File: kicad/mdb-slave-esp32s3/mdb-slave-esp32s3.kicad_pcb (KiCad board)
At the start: 2 copper layers, 39 x 40 mm, 45 parts, among them J1 MDB_Connector, J2 USB_C_Receptacle_USB2.0_16P, J3 Conn_01x03_Pin, J8 Conn_01x04_Pin, Q7 MMBT3904, SW1 SW_Push, U1 TLP785, U3 ESP32-S3FH4R2, U4 TLP785, U5 LM2594HVM-3.3, Y1 Crystal_GND24

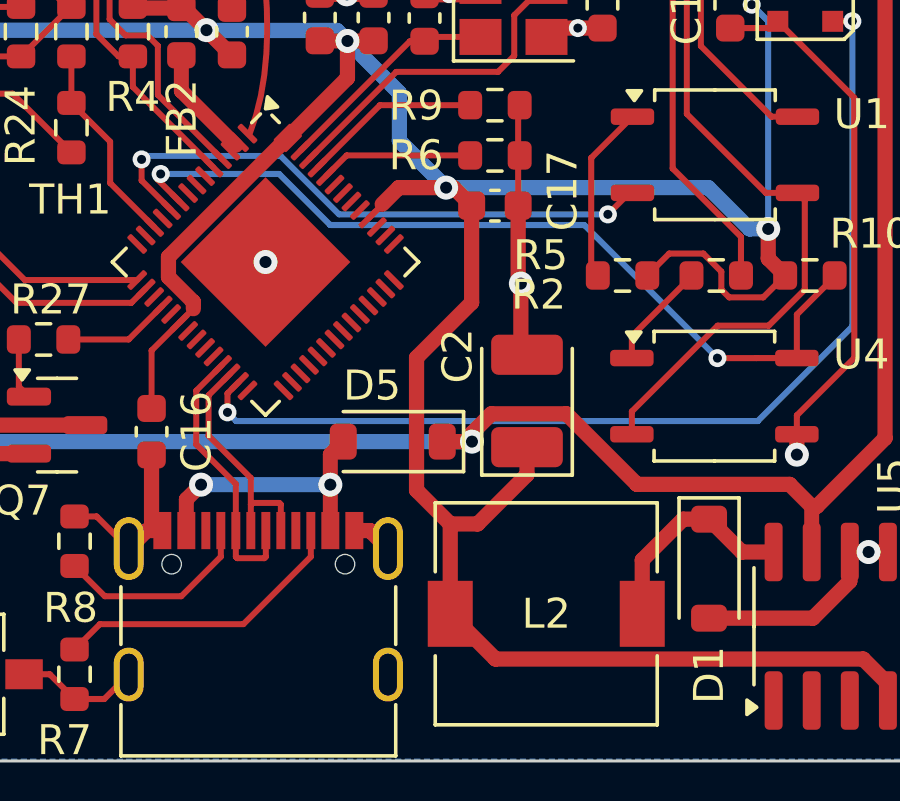
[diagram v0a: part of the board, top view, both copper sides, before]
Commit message: routing...
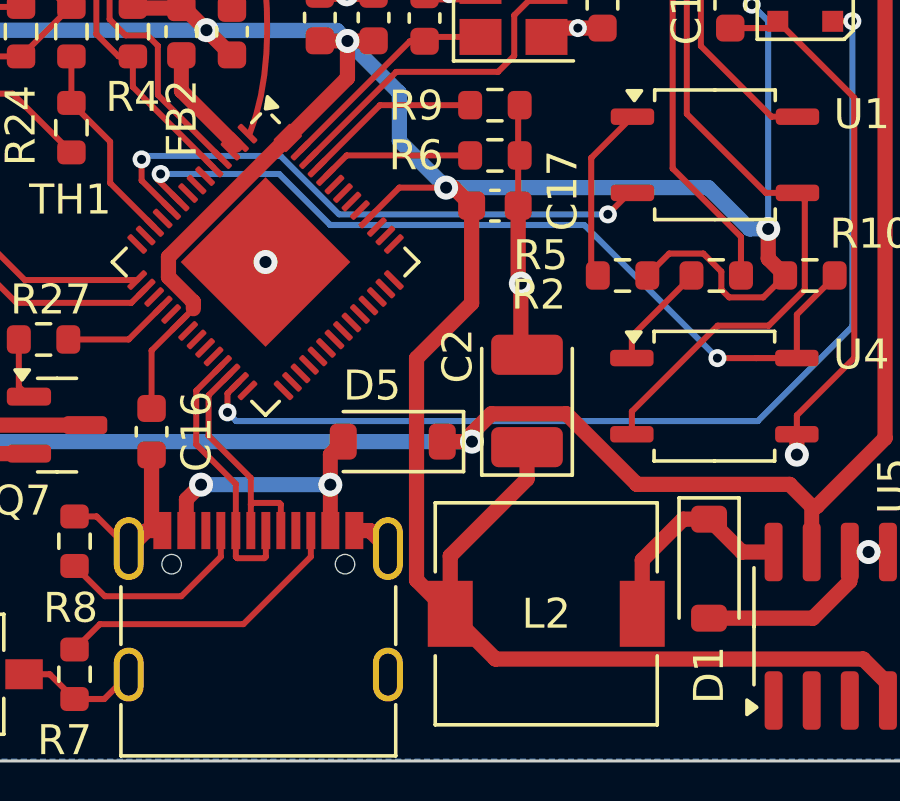
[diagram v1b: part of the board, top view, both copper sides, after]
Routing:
- net +3V3: track 125.0 -> 127.4 mm
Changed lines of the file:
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@@
+	)
+	(segment
+		(start 194.325 112.63)
+		(end 194.325 113.695)
+		(width 0.508)
+		(layer "F.Cu")
+		(net 2)
 	)
 	(segment
@@
 	)
 	(segment
-		(start 189.496806 104.550048)
-		(end 189.038427 105.008427)
-		(width 0.2032)
-		(layer "F.Cu")
-		(net 2)
-	)
-	(segment
 		(start 200.201177 106.176875)
 		(end 200.802167 106.777865)
@@
 	)
 	(segment
-		(start 192.48 107.81)
-		(end 190.6426 109.6474)
+		(start 194.325 113.695)
+		(end 191.766 116.254)
 		(width 0.508)
 		(layer "F.Cu")
@@
 	)
 	(segment
+		(start 192.48 107.83)
+		(end 192.48 104.58)
+		(width 0.508)
+		(layer "F.Cu")
+		(net 2)
+	)
+	(segment
+		(start 191.628427 103.978427)
+		(end 190.068427 103.978427)
+		(width 0.2032)
+		(layer "F.Cu")
+		(net 2)
+	)
+	(segment
 		(start 177.46 99.605)
 		(end 176.035 99.605)
@@
 	)
 	(segment
-		(start 192.48 104.58)
+		(start 190.6426 109.6674)
+		(end 192.48 107.83)
+		(width 0.508)
+		(layer "F.Cu")
+		(net 2)
+	)
+	(segment
+		(start 191.628427 103.978427)
 		(end 191.878427 103.978427)
 		(width 0.508)
@@
 		(end 202.2 107.636875)
 		(width 0.2032)
-		(layer "F.Cu")
-		(net 2)
-	)
-	(segment
-		(start 191.766 115.189)
-		(end 191.766 118.185)
-		(width 0.508)
 		(layer "F.Cu")
 		(net 2)
@@
 	)
 	(segment
-		(start 192.681 115.189)
-		(end 191.766 115.189)
+		(start 191.878427 103.978427)
+		(end 192.48 104.58)
 		(width 0.508)
 		(layer "F.Cu")
@@
 	)
 	(segment
-		(start 190.6426 109.6474)
-		(end 190.6426 114.0656)
-		(width 0.508)
-		(layer "F.Cu")
-		(net 2)
-	)
-	(segment
 		(start 202.2 107.636875)
 		(end 202.93 106.906875)
@@
 	)
 	(segment
+		(start 191.766 116.254)
+		(end 191.766 118.185)
+		(width 0.508)
+		(layer "F.Cu")
+		(net 2)
+	)
+	(segment
 		(start 179.138333 97.955)
 		(end 179.11 97.955)
 		(width 0.2)
-		(layer "F.Cu")
-		(net 2)
-	)
-	(segment
-		(start 191.878427 103.978427)
-		(end 190.051573 103.978427)
-		(width 0.508)
 		(layer "F.Cu")
 		(net 2)
@@
 	)
 	(segment
+		(start 190.068427 103.978427)
+		(end 189.038427 105.008427)
+		(width 0.2032)
+		(layer "F.Cu")
+		(net 2)
+	)
+	(segment
+		(start 190.6426 117.0616)
+		(end 190.6426 109.6674)
+		(width 0.508)
+		(layer "F.Cu")
+		(net 2)
+	)
+	(segment
 		(start 205.5324 119.6924)
 		(end 206.355 120.515)
@@
 	)
 	(segment
-		(start 194.325 112.63)
-		(end 194.325 113.545)
-		(width 0.508)
-		(layer "F.Cu")
-		(net 2)
-	)
-	(segment
-		(start 190.6426 114.0656)
-		(end 191.766 115.189)
-		(width 0.508)
-		(layer "F.Cu")
-		(net 2)
-	)
-	(segment
 		(start 177.46 96.505)
 		(end 177.545 96.505)
@@
 	)
 	(segment
+		(start 191.766 118.185)
+		(end 190.6426 117.0616)
+		(width 0.508)
+		(layer "F.Cu")
+		(net 2)
+	)
+	(segment
 		(start 200.802167 107.375885)
 		(end 201.063157 107.636875)
@@
 	)
 	(segment
-		(start 194.325 113.545)
-		(end 192.681 115.189)
-		(width 0.508)
-		(layer "F.Cu")
-		(net 2)
-	)
-	(segment
 		(start 179.11 97.955)
 		(end 177.46 99.605)
@@
 		(end 178.995 97.955)
 		(width 0.2)
-		(layer "F.Cu")
-		(net 2)
-	)
-	(segment
-		(start 192.48 104.58)
-		(end 192.48 107.81)
-		(width 0.508)
 		(layer "F.Cu")
 		(net 2)
@@
 	)
 	(segment
-		(start 189.496806 104.533194)
-		(end 189.496806 104.550048)
-		(width 0.2032)
-		(layer "F.Cu")
-		(net 2)
-	)
-	(segment
 		(start 176.035 99.605)
 		(end 175.276667 98.846667)
 		(width 0.2)
-		(layer "F.Cu")
-		(net 2)
-	)
-	(segment
-		(start 190.051573 103.978427)
-		(end 189.496806 104.533194)
-		(width 0.508)
 		(layer "F.Cu")
 		(net 2)
@@
 		(name "$teardrop_padvia$")
 		(hatch none 0.1)
-		(priority 30000)
+		(priority 30015)
 		(attr
 			(teardrop
@@
 		(polygon
 			(pts
-				(xy 194.101332 84.372878) (xy 193.742122 84.013668) (xy 192.339088 84.361698) (xy 192.124293 85.990707)
-				(xy 193.475 86.054213)
+				(xy 180.192157 120.9234) (xy 180.192157 121.1266) (xy 180.872955 121.067877) (xy 181.05 120.21)
+				(xy 180.549 119.996303)
 			)
 		)
 	)
 	(zone
-		(net 3)
-		(net_name "GND")
+		(net 27)
+		(net_name "/io11")
 		(layer "F.Cu")
 		(name "$teardrop_padvia$")
 		(hatch none 0.1)
-		(priority 30001)
+		(priority 30008)
 		(attr
 			(teardrop
@@
 		(polygon
 			(pts
-				(xy 190.507878 84.013668) (xy 190.148668 84.372878) (xy 190.775 86.054213) (xy 192.125707 85.990707)
-				(xy 191.910911 84.361698)
+				(xy 172.109084 95.731162) (xy 172.250505 95.872583) (xy 173.383528 95.446667) (xy 173.135707 94.84596)
+				(xy 172.271529 94.861609)
 			)
 		)
@@
 		(name "$teardrop_padvia$")
 		(hatch none 0.1)
-		(priority 30014)
+		(priority 30007)
 		(attr
 			(teardrop
@@
 		(polygon
 			(pts
-				(xy 180.267289 115.084605) (xy 180.123605 115.228289) (xy 180.549 116.217106) (xy 181.049707 116.010707)
-				(xy 180.78476 115.038654)
+				(xy 174.61 100.948267) (xy 174.61 100.745067) (xy 173.855671 100.265697) (xy 173.134 100.846667)
+				(xy 173.855671 101.427637)
 			)
 		)
@@
 		(name "$teardrop_padvia$")
 		(hatch none 0.1)
-		(priority 30011)
+		(priority 30006)
 		(attr
 			(teardrop
@@
 		(polygon
 			(pts
-				(xy 174.598471 96.946667) (xy 174.598471 96.746667) (xy 173.743342 96.347785) (xy 173.134 96.846667)
-				(xy 173.743342 97.345549)
+				(xy 171.92558 97.592999) (xy 172.067001 97.73442) (xy 173.327746 97.446667) (xy 173.135707 96.84596)
+				(xy 172.271529 96.729613)
 			)
 		)
@@
 		(name "$teardrop_padvia$")
 		(hatch none 0.1)
-		(priority 30007)
+		(priority 30013)
 		(attr
 			(teardrop
@@
 		(polygon
 			(pts
-				(xy 174.61 100.948267) (xy 174.61 100.745067) (xy 173.855671 100.265697) (xy 173.134 100.846667)
-				(xy 173.855671 101.427637)
+				(xy 188.730421 115.156) (xy 188.730421 115.664) (xy 189.189 116.286434) (xy 189.69 116.01) (xy 189.287099 115.16838)
 			)
 		)
@@
 	)
 	(zone
-		(net 27)
-		(net_name "/io11")
+		(net 12)
+		(net_name "/mdb_master_receive")
 		(layer "F.Cu")
 		(name "$teardrop_padvia$")
 		(hatch none 0.1)
-		(priority 30008)
+		(priority 30003)
 		(attr
 			(teardrop
@@
 		(polygon
 			(pts
-				(xy 172.109084 95.731162) (xy 172.250505 95.872583) (xy 173.383528 95.446667) (xy 173.135707 94.84596)
-				(xy 172.271529 94.861609)
+				(xy 189.792438 89.763983) (xy 189.651017 89.622562) (xy 188.139088 89.861698) (xy 187.924293 91.490707)
+				(xy 189.275 91.554214)
 			)
 		)
 	)
 	(zone
-		(net 27)
-		(net_name "/io11")
+		(net 2)
+		(net_name "+3V3")
 		(layer "F.Cu")
 		(name "$teardrop_padvia$")
 		(hatch none 0.1)
-		(priority 30009)
+		(priority 30010)
 		(attr
 			(teardrop
@@
 		(polygon
 			(pts
-				(xy 174.598471 94.946667) (xy 174.598471 94.746667) (xy 173.743342 94.347785) (xy 173.134 94.846667)
-				(xy 173.743342 95.345549)
+				(xy 174.598471 98.946667) (xy 174.598471 98.746667) (xy 173.743342 98.347785) (xy 173.134 98.846667)
+				(xy 173.743342 99.345549)
 			)
 		)
 	)
 	(zone
-		(net 23)
-		(net_name "/io10")
+		(net 3)
+		(net_name "GND")
 		(layer "F.Cu")
 		(name "$teardrop_padvia$")
 		(hatch none 0.1)
-		(priority 30006)
+		(priority 30012)
 		(attr
 			(teardrop
@@
 		(polygon
 			(pts
-				(xy 171.92558 97.592999) (xy 172.067001 97.73442) (xy 173.327746 97.446667) (xy 173.135707 96.84596)
-				(xy 172.271529 96.729613)
+				(xy 182.007579 115.664) (xy 182.007579 115.156) (xy 181.4509 115.16838) (xy 181.048 116.01) (xy 181.549 116.286434)
 			)
 		)
 	)
 	(zone
-		(net 2)
-		(net_name "+3V3")
+		(net 3)
+		(net_name "GND")
 		(layer "F.Cu")
 		(name "$teardrop_padvia$")
 		(hatch none 0.1)
-		(priority 30010)
+		(priority 30001)
 		(attr
 			(teardrop
@@
 		(polygon
 			(pts
-				(xy 174.598471 98.946667) (xy 174.598471 98.746667) (xy 173.743342 98.347785) (xy 173.134 98.846667)
-				(xy 173.743342 99.345549)
+				(xy 190.507878 84.013668) (xy 190.148668 84.372878) (xy 190.775 86.054213) (xy 192.125707 85.990707)
+				(xy 191.910911 84.361698)
 			)
 		)
@@
 		(name "$teardrop_padvia$")
 		(hatch none 0.1)
-		(priority 30012)
+		(priority 30000)
 		(attr
 			(teardrop
@@
 		(polygon
 			(pts
-				(xy 182.007579 115.664) (xy 182.007579 115.156) (xy 181.4509 115.16838) (xy 181.048 116.01) (xy 181.549 116.286434)
+				(xy 194.101332 84.372878) (xy 193.742122 84.013668) (xy 192.339088 84.361698) (xy 192.124293 85.990707)
+				(xy 193.475 86.054213)
 			)
 		)
 	)
 	(zone
-		(net 3)
-		(net_name "GND")
+		(net 23)
+		(net_name "/io10")
 		(layer "F.Cu")
 		(name "$teardrop_padvia$")
 		(hatch none 0.1)
-		(priority 30013)
+		(priority 30011)
 		(attr
 			(teardrop
@@
 		(polygon
 			(pts
-				(xy 188.730421 115.156) (xy 188.730421 115.664) (xy 189.189 116.286434) (xy 189.69 116.01) (xy 189.287099 115.16838)
+				(xy 174.598471 96.946667) (xy 174.598471 96.746667) (xy 173.743342 96.347785) (xy 173.134 96.846667)
+				(xy 173.743342 97.345549)
 			)
 		)
 	)
 	(zone
-		(net 3)
-		(net_name "GND")
+		(net 27)
+		(net_name "/io11")
 		(layer "F.Cu")
 		(name "$teardrop_padvia$")
 		(hatch none 0.1)
-		(priority 30015)
+		(priority 30009)
 		(attr
 			(teardrop
@@
 		(polygon
 			(pts
-				(xy 180.192157 120.9234) (xy 180.192157 121.1266) (xy 180.872955 121.067877) (xy 181.05 120.21)
-				(xy 180.549 119.996303)
+				(xy 174.598471 94.946667) (xy 174.598471 94.746667) (xy 173.743342 94.347785) (xy 173.134 94.846667)
+				(xy 173.743342 95.345549)
 			)
 		)
 	)
 	(zone
-		(net 12)
-		(net_name "/mdb_master_receive")
+		(net 3)
+		(net_name "GND")
 		(layer "F.Cu")
 		(name "$teardrop_padvia$")
 		(hatch none 0.1)
-		(priority 30003)
+		(priority 30014)
 		(attr
 			(teardrop
@@
 		(polygon
 			(pts
-				(xy 189.792438 89.763983) (xy 189.651017 89.622562) (xy 188.139088 89.861698) (xy 187.924293 91.490707)
-				(xy 189.275 91.554214)
-			)
-		)
+				(xy 180.267289 115.084605) (xy 180.123605 115.228289) (xy 180.549 116.217106) (xy 181.049707 116.010707)
+				(xy 180.78476 115.038654)
+			)
+		)
